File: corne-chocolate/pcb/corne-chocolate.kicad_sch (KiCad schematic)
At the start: 83 parts, among them J1 MJ-4PP-9, J2 Conn_01x04, J3 Conn_01x03, P1 Conn_01x01, P2 Conn_01x01, SW1 SW_PUSH, SW10 SW_PUSH, SW11 SW_PUSH, SW12 SW_PUSH, SW13 SW_PUSH, SW14 SW_PUSH, SW15 SW_PUSH, SW16 SW_PUSH, SW17 SW_PUSH, SW18 SW_PUSH, SW19 SW_PUSH, SW2 SW_PUSH, SW20 SW_PUSH, SW21 SW_PUSH, SW3 SW_PUSH, SW4 SW_PUSH, SW5 SW_PUSH, SW6 SW_PUSH, SW7 SW_PUSH, SW8 SW_PUSH, SW9 SW_PUSH, U1 ProMicro

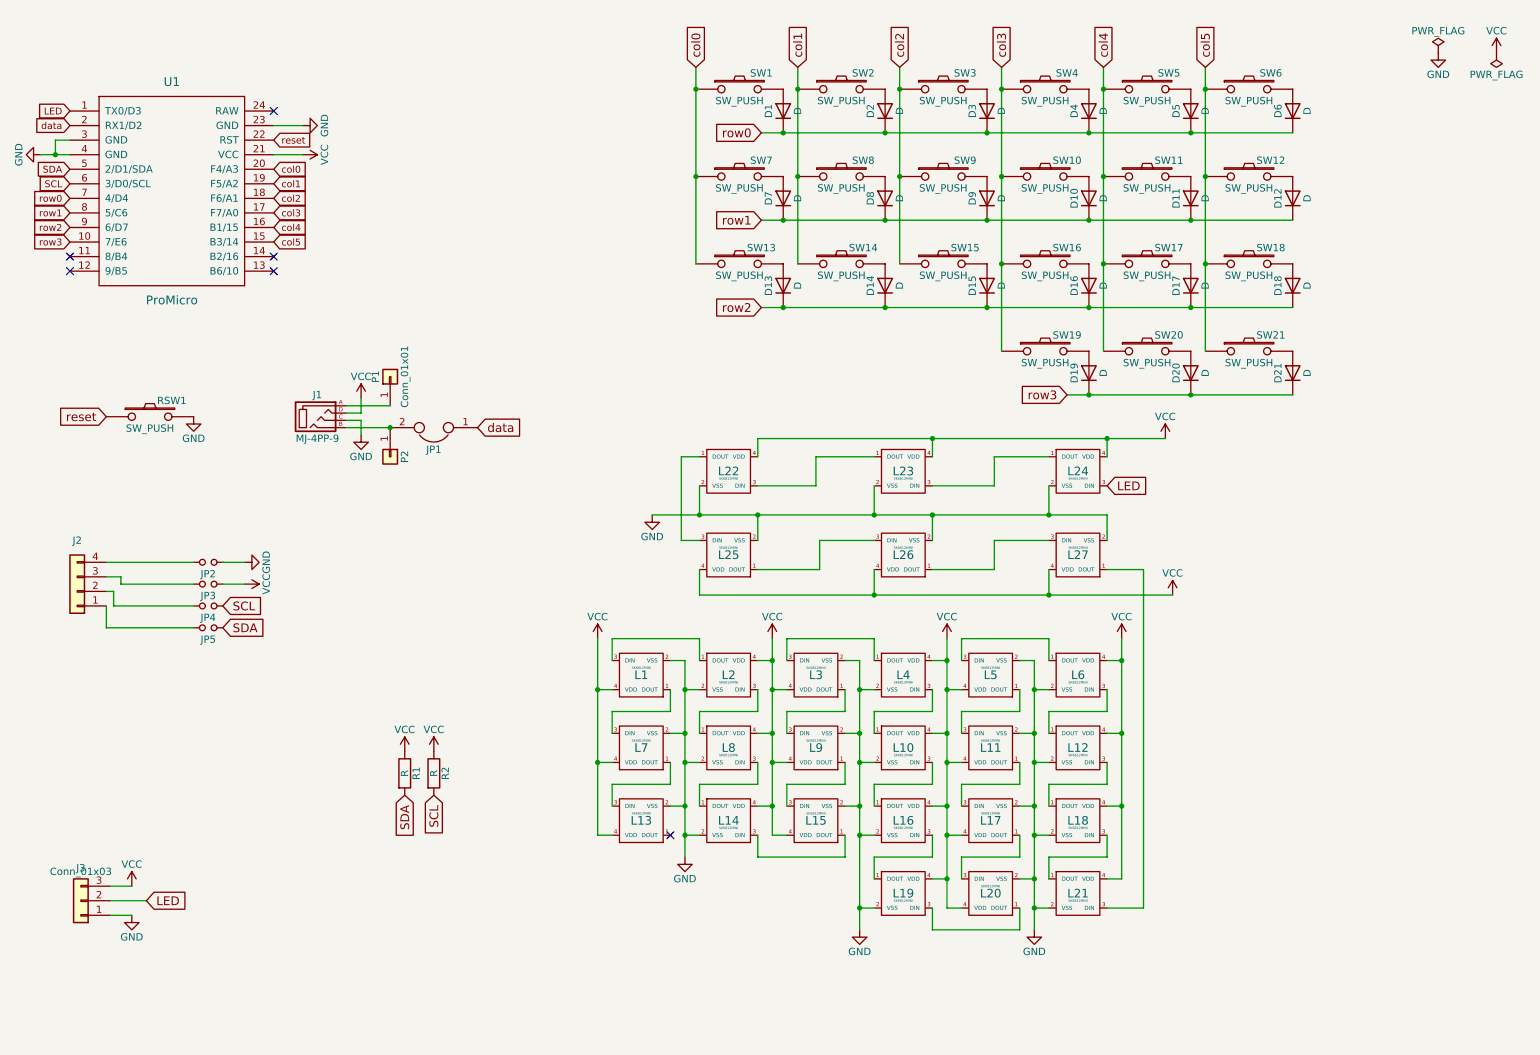
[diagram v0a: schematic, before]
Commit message: starts re-routing. switch to a 3x5 kbd
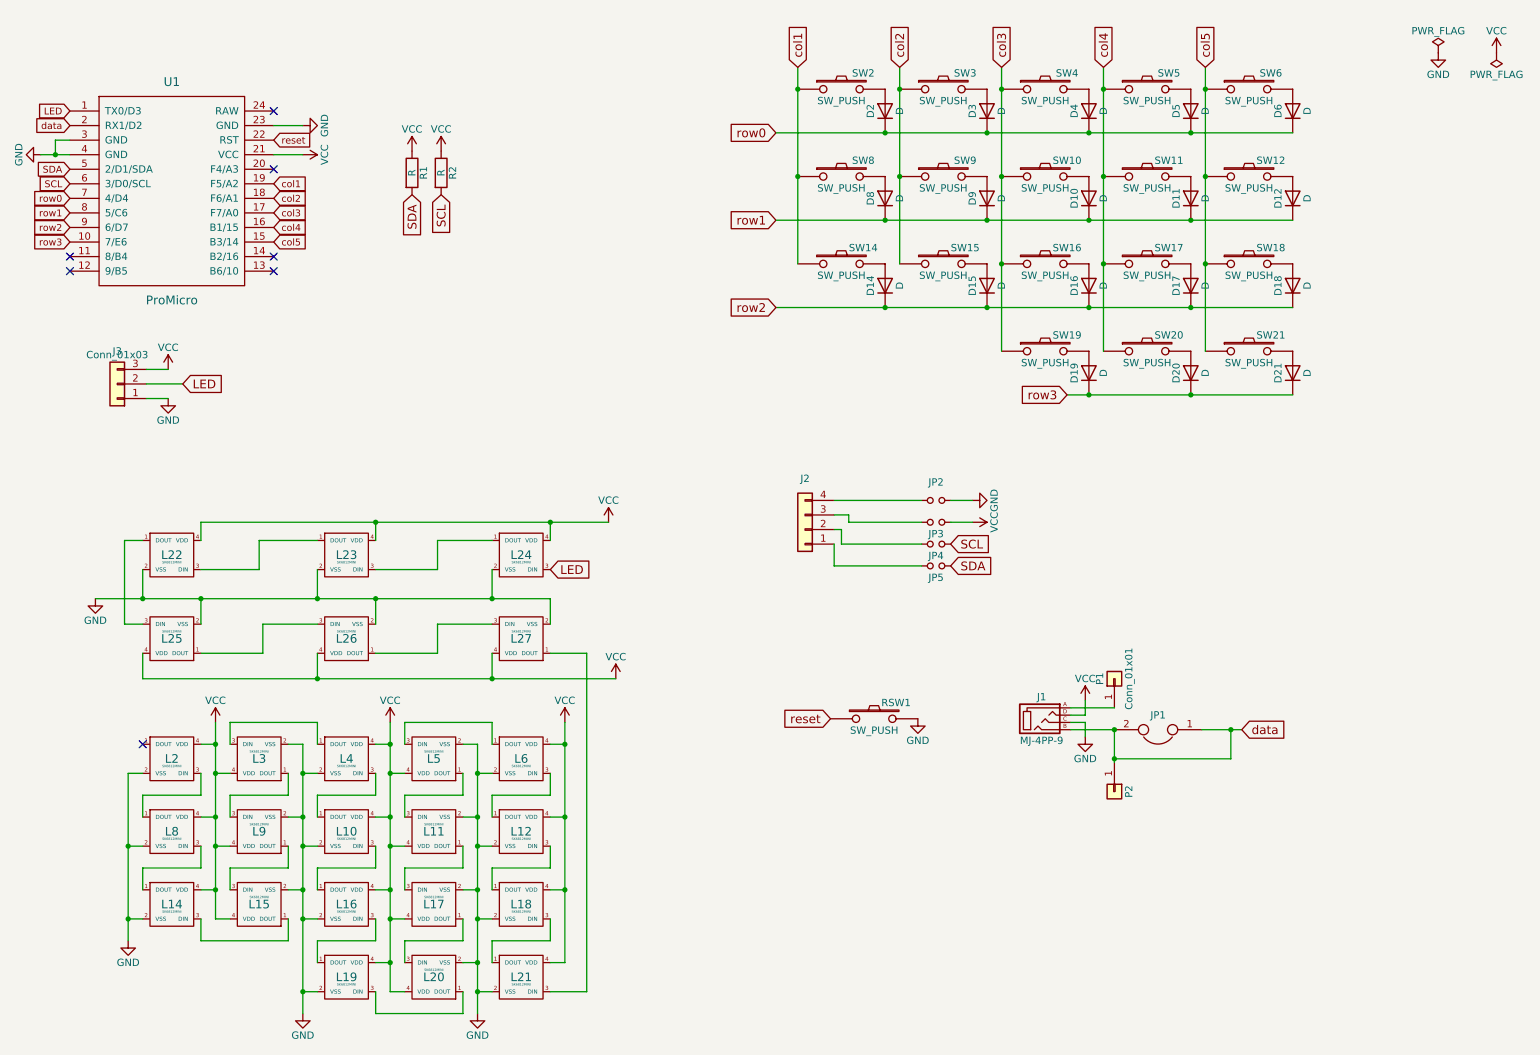
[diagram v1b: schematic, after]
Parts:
- removed D1, D13, D7: D, kbd:D3_SMD, symbol Device:D
- removed L1, L13, L7: SK6812MINI, kbd:SK6812MINI_rev, symbol kbd:SK6812MINI
- removed SW1, SW13, SW7: SW_PUSH, kbd:ChocV1_V2_Hotswap, symbol kbd:SW_PUSH
- JP1: footprint kbd:JPC2 -> kbd:Jumper
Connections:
- net GND: now also JP2.2; no longer JP2.1
- net data: now also J1.B, JP1.2, P2.1 (Pin_1)
- net at J2.4 (Pin_4): now also JP2.1; no longer JP2.2
- net col0: no longer names the net of U1.20 (F4/A3)
- no-connect marks 6 -> 7
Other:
- moved on the sheet: J1, J2, J3, JP3, JP4, JP5, L10, L11, L12, L14, L15, L16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
